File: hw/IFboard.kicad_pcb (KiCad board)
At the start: 2 copper layers, 105 x 65.1 mm, 99 parts, among them J1 USB_C_Receptacle_USB2.0_16P, J10 Conn_01x01_MountingPin, J2 Conn_01x03_Socket, J3 Conn_ARM_SWD_TagConnect_TC203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, J4 Conn_01x03_Socket, J5 Conn_01x03_Socket, J6 Conn_01x03_Socket, J7 Conn_01x01_MountingPin, J8 Conn_01x01_MountingPin, J9 Conn_01x01_MountingPin, SW3 SW_Push, SW4 SW_Push, SW5 SW_Push, SW6 SW_Push, U2 XC6206PxxxMR, U3 TCAN3413DR, U4 ST4E1240DT, U5 MAX232ESE+T, U6 STM32G0B1CBTx, U7 ER_OLEDM0.91_1x-I2C

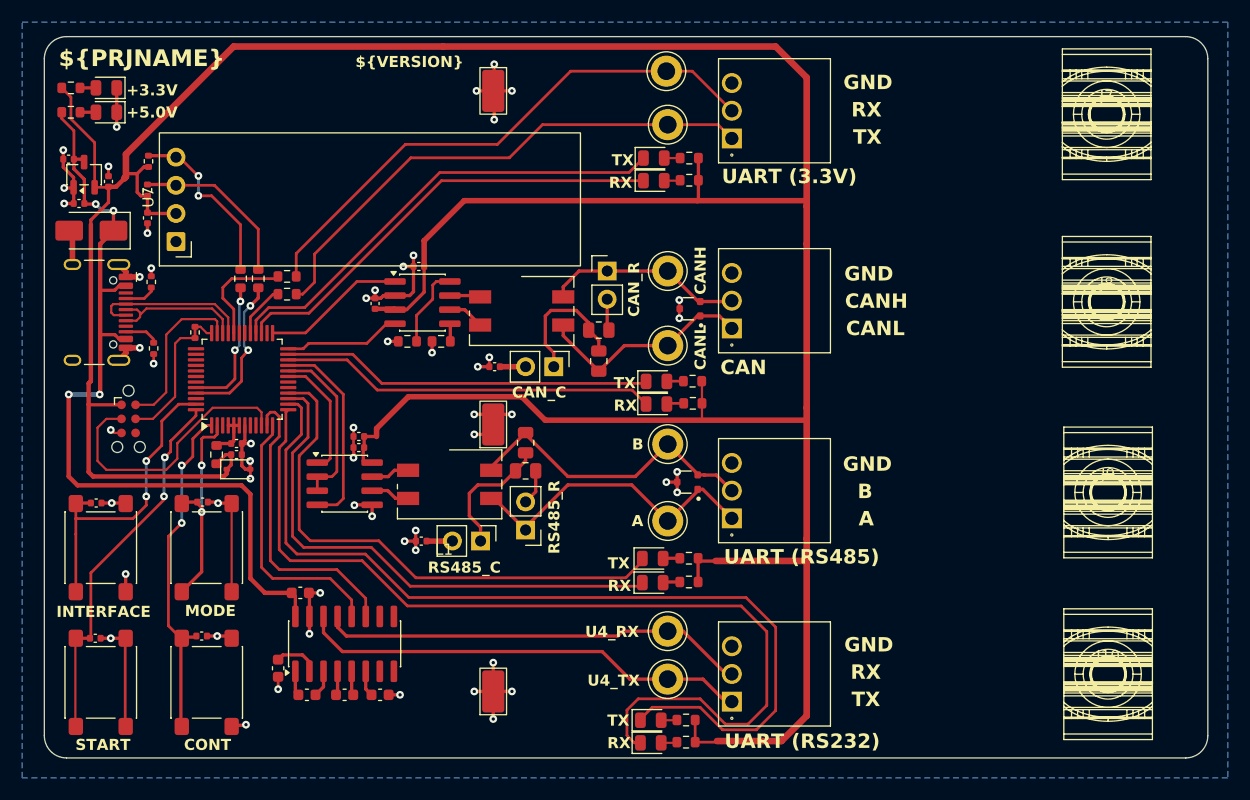
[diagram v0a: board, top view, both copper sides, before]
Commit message: cleanup
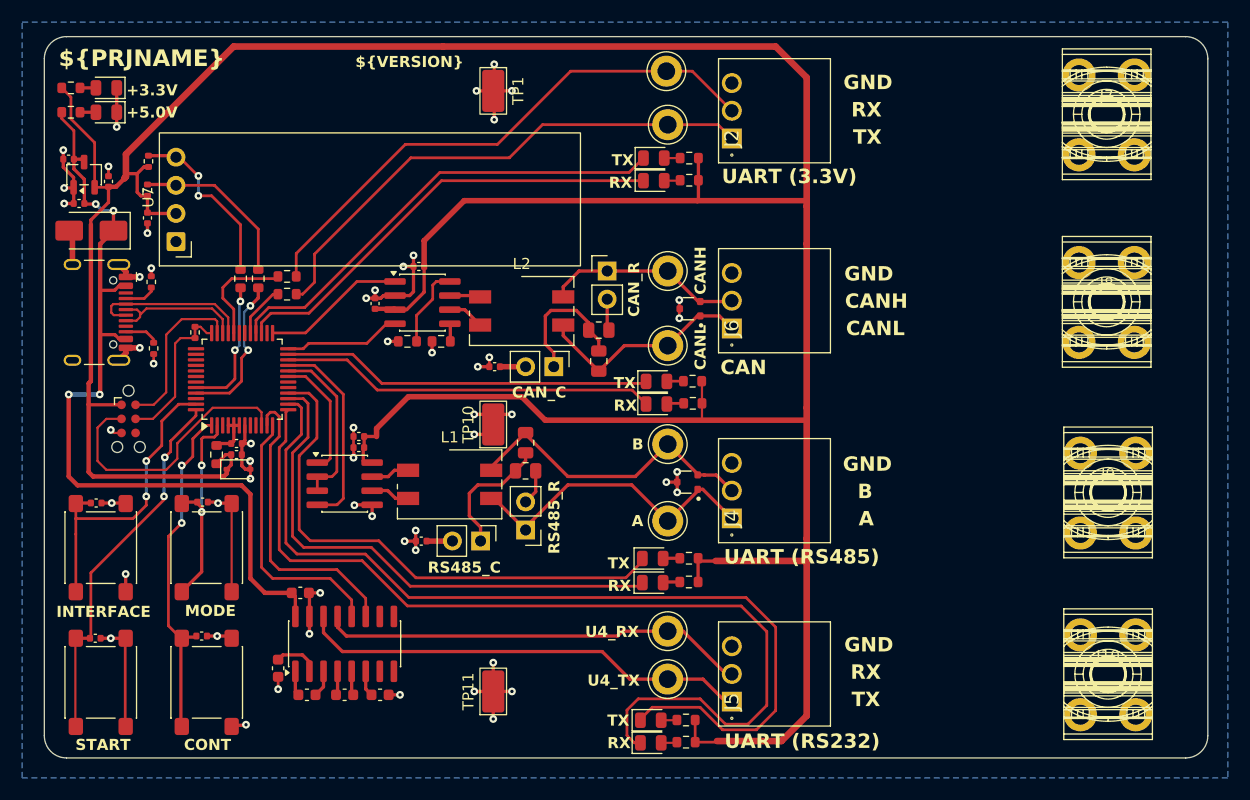
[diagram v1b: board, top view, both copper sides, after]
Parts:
- J10, J7, J8, J9: value Conn_01x01_MountingPin -> IcoTec_36650.2; footprint Connector_PinHeader_1.00mm:PinHeader_1x01_P1.00mm_Vertical -> PZ:icotek 36650.2 PCB-4-V-6,8SKL 3-6
- U2: value XC6206PxxxMR -> XC6206P332MR-G
